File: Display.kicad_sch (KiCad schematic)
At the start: 5 parts

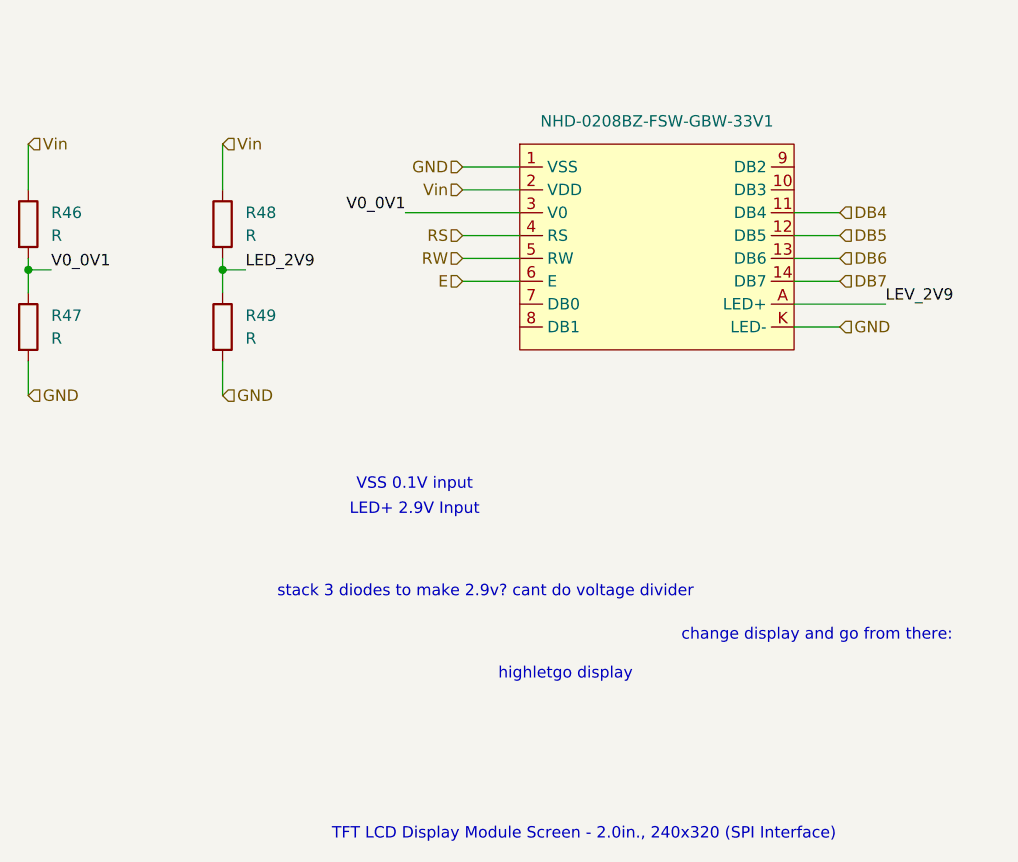
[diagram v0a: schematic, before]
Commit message: schematic1
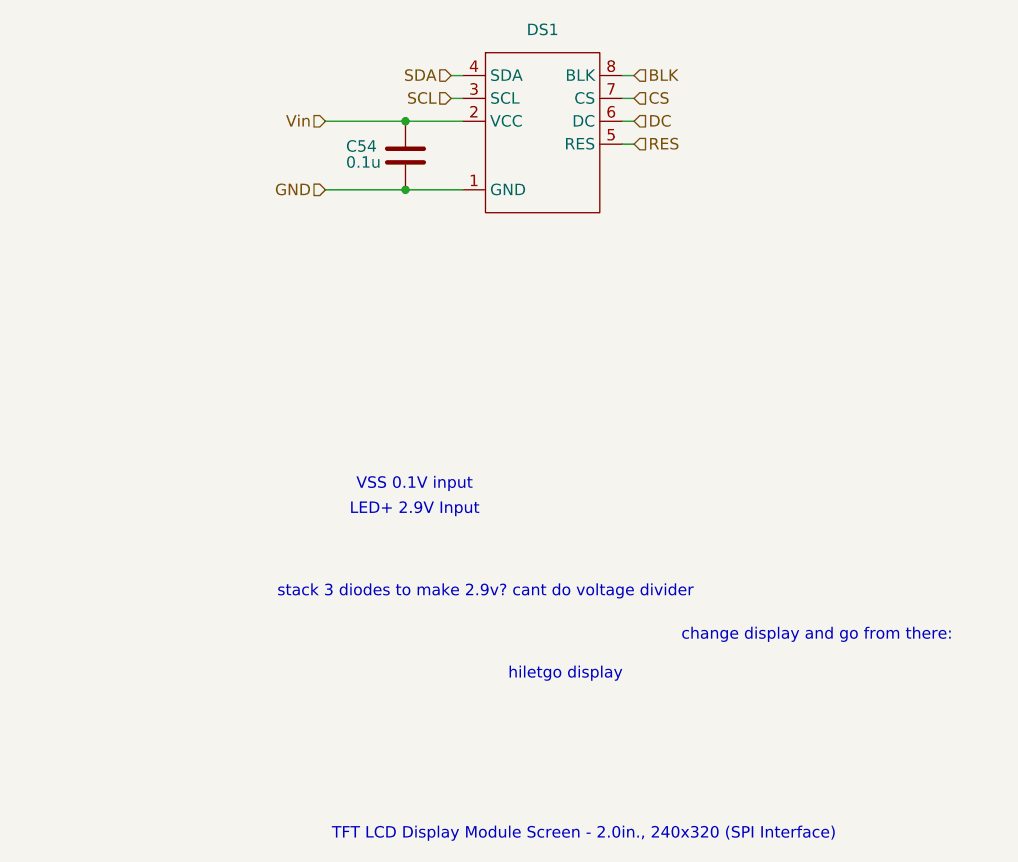
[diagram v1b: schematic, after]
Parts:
- removed NHD-0208BZ-FSW-GBW-33V1: (no value), symbol PS-SuppCharger_Library:NHD-0208BZ-FSW-GBW-33V3
- removed R46, R47, R48, R49: R, symbol Device:R
- added C54: 0.1u, symbol Device:C
- added DS1: (no value), symbol PS-SuppCharger_Library:ZJY200S0800TG01
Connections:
- net GND: now also C54.2, DS1.1 (GND)
- net Vin: now also C54.1, DS1.2 (VCC)
- new net BLK: DS1.8 (BLK)
- new net CS: DS1.7 (CS)
- new net DC: DS1.6 (DC)
- new net RES: DS1.5 (RES)
- new net SCL: DS1.3 (SCL)
- new net SDA: DS1.4 (SDA)
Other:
- note added: "hiletgo display"
- note removed: "highletgo display"
